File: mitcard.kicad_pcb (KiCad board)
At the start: 2 copper layers, 91 x 55 mm, 14 parts, among them J1 MJ-4PP-9, J2 MJ-4PP-9, J3 Conn_01x08, SW1 SW_PUSH, SW2 SW_PUSH, SW3 SW_PUSH, SW4 SW_PUSH, U1 Teensy-LC

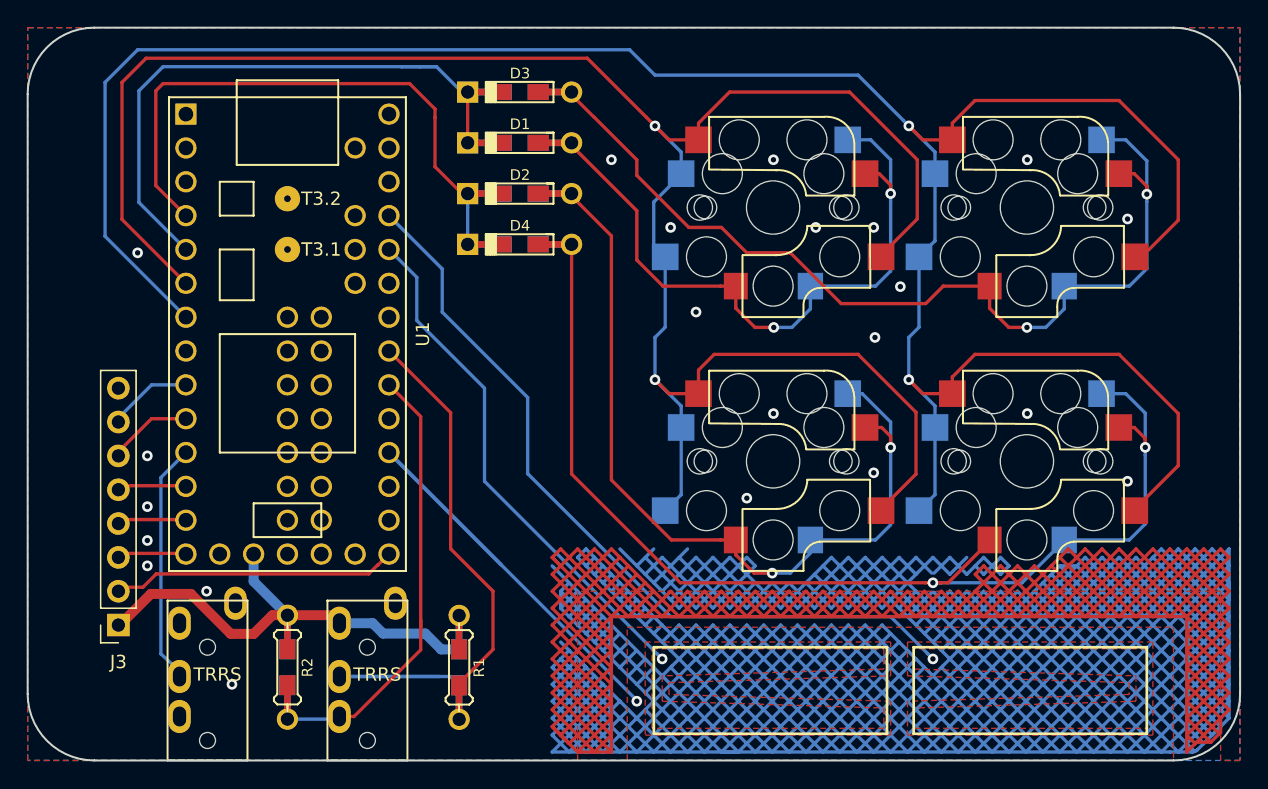
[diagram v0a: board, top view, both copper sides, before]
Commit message: 足の置き場を確保
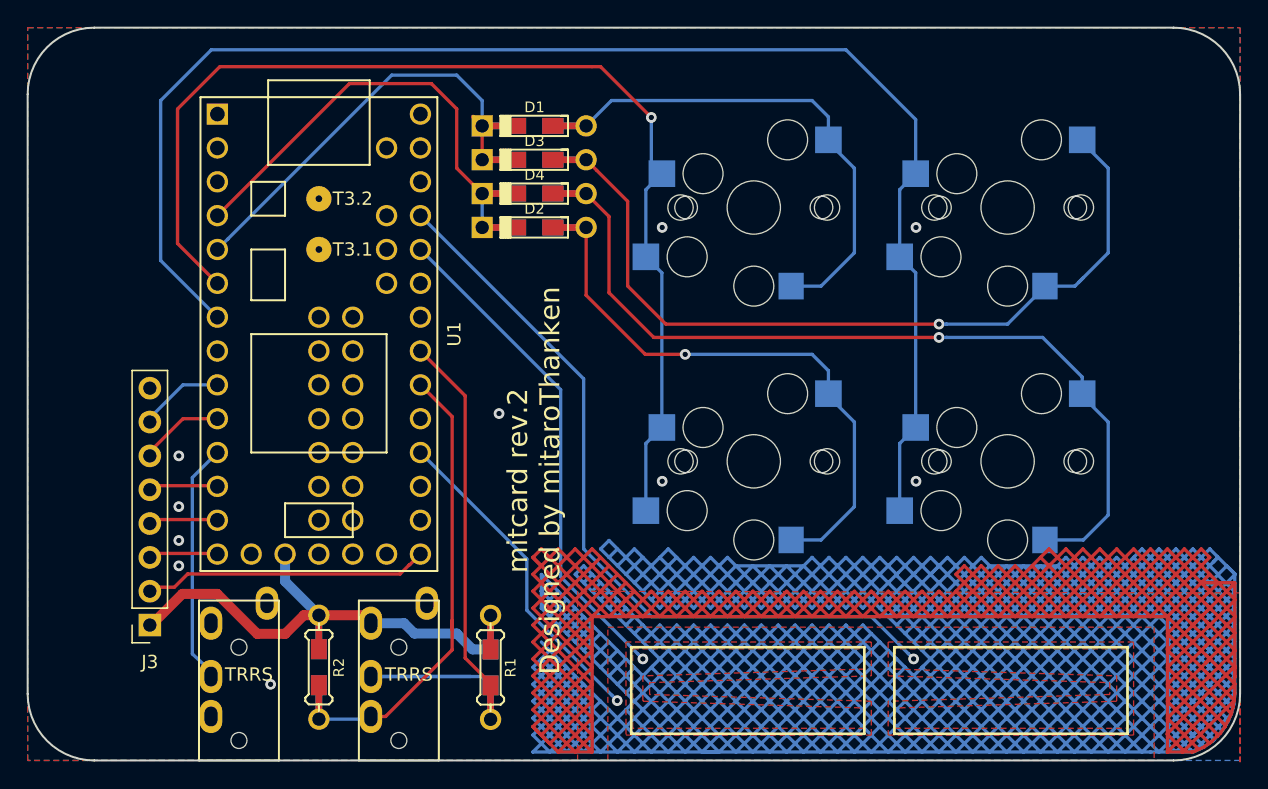
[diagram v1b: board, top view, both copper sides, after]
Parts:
- SW1, SW2, SW3, SW4: footprint kbd:CherryMX_Choc_Hotswap -> kbd:CherryMX_Choc_Hotswap_1side
- moved D3 5.20 mm to (88.0, 59.9)
- moved D4 3.96 mm to (88.0, 62.5)
- moved D2 2.76 mm to (88.0, 65.0)
- moved J1 2.36 mm to (77.9, 105.0)
- moved J2 2.36 mm to (65.9, 105.0)
- moved J3 2.36 mm to (59.2, 94.8)
- moved R1 2.36 mm to (84.7, 98.0)
- moved R2 2.36 mm to (71.9, 98.0)
- moved U1 2.36 mm to (71.9, 73.0)
- moved D1 1.67 mm to (88.0, 57.4)
- moved SW1 1.45 mm to (104.5, 63.5)
- moved SW2 1.45 mm to (104.5, 82.5)
- moved SW3 1.45 mm to (123.5, 63.5)
- moved SW4 1.45 mm to (123.5, 82.5)
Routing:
- net GND: track 2139.7 -> 2334.6 mm, vias 22 -> 10
- net col0: track 158.2 -> 84.5 mm, vias 2 -> 1
- net col1: track 182.1 -> 109.3 mm, vias 2 -> 0
- net Net-(D4-Pad2): track 85.7 -> 63.0 mm, vias 2 -> 1
- net Net-(D2-Pad2): track 64.6 -> 42.4 mm, vias 2 -> 1
- net row0: track 47.6 -> 30.7 mm
- net Net-(D1-Pad2): track 52.2 -> 36.8 mm, vias 2 -> 0
- net Net-(U1-Pad23): track 38.3 -> 24.7 mm
- net /col1row0: track 73.2 -> 59.9 mm, vias 2 -> 1
- net row1: track 45.4 -> 32.5 mm
- net /SCL: track 48.1 -> 46.0 mm
- net Net-(U1-Pad29): track 39.2 -> 37.6 mm
- net Net-(U1-Pad30): track 59.9 -> 58.3 mm
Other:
- board text added: "mitcard rev.2 Designed by mitaroThanken"
- board text removed: "mitcard rev.1 Designed by mitaroThanken"
